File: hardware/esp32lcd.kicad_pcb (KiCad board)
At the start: 2 copper layers, 78 x 44 mm, 25 parts, among them J1 Conn_02x05_Odd_Even, J11 USB_B_Micro, J12 Barrel_Jack_Switch, Q1 MMBT5551, Q12 MMBT5551, Q13 MMBT5401, U11 SRV05-4, U12 CH340C, U13 AMS1117-3.3, U14 ESP32-WROOM-32D, U15 ILI9341_SPI_Touch_SD

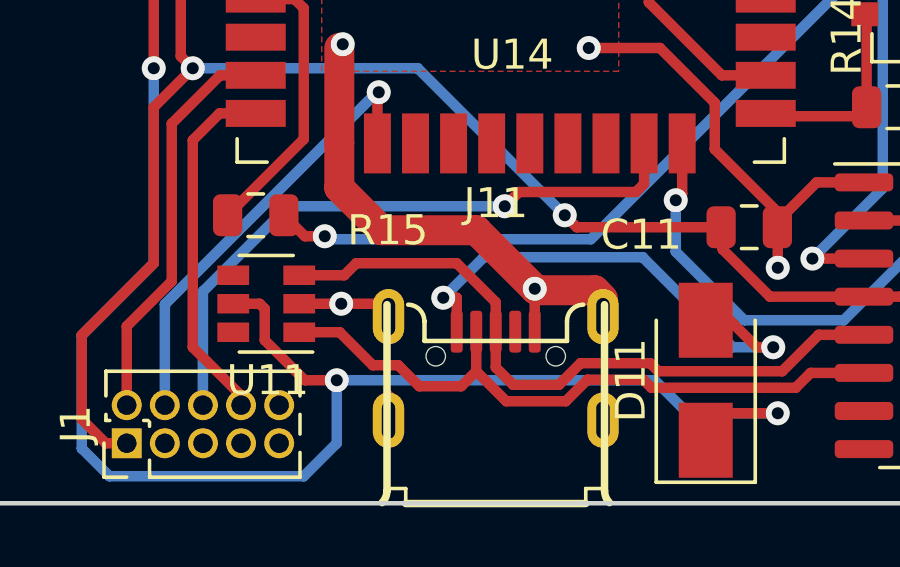
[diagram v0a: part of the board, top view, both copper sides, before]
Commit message: Last version before moving to Kicad10 and JLC Basic/Extended libraries
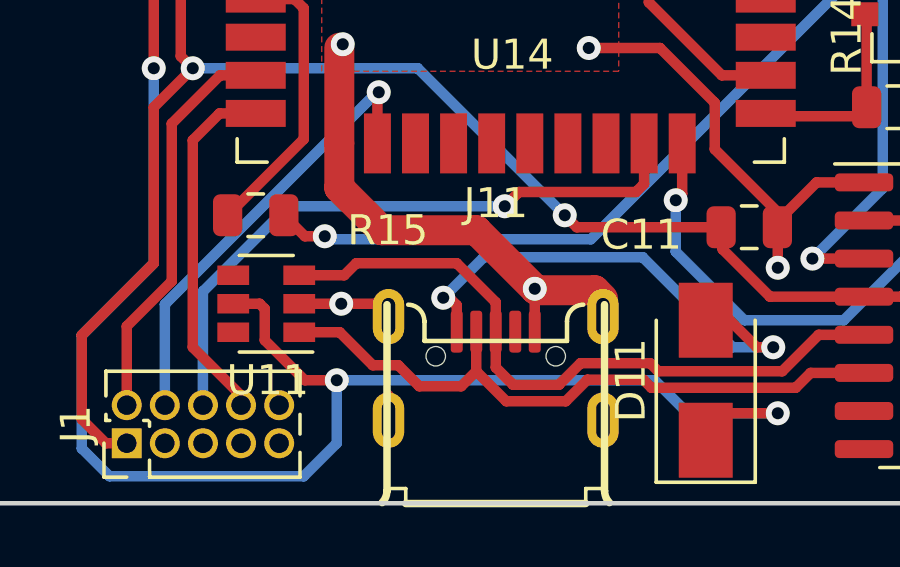
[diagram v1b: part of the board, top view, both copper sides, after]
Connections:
- net /RXD0 renamed RXD0
- net /TXD0 renamed TXD0
- net Net-(Q1-Pad3) renamed LOAD
- net Net-(U14-Pad27) renamed RXD2
- net Net-(U14-Pad28) renamed TXD2
- Q13 pad 3: BACKLIGHT -> LCDLED
- R15 pad 1: Net-(R15-Pad1) -> BACKLIGHT
- U14 pad 11: Net-(R15-Pad1) -> BACKLIGHT
- U15 pad 8: BACKLIGHT -> LCDLED
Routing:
- net LCDLED: track 0.00 -> 17.7 mm, vias 0 -> 1
- net Net-(R15-Pad1): track 9.68 -> 0.00 mm
- net BACKLIGHT: track 17.7 -> 9.68 mm, vias 1 -> 0
